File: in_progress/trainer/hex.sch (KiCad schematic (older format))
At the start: 46 parts, among them IC1 ATMEGA16-P, P12 CONN_02X08, P13 CONN_01X02, Q2 2N3904, Q3 2N3904, Q4 2N3904, Q5 2N3904, SW22 DEC/HEX, SW23 SW_PUSH, SW24 SW_PUSH, U10 JHD-162A, U8 4067, U9 ULN2803A

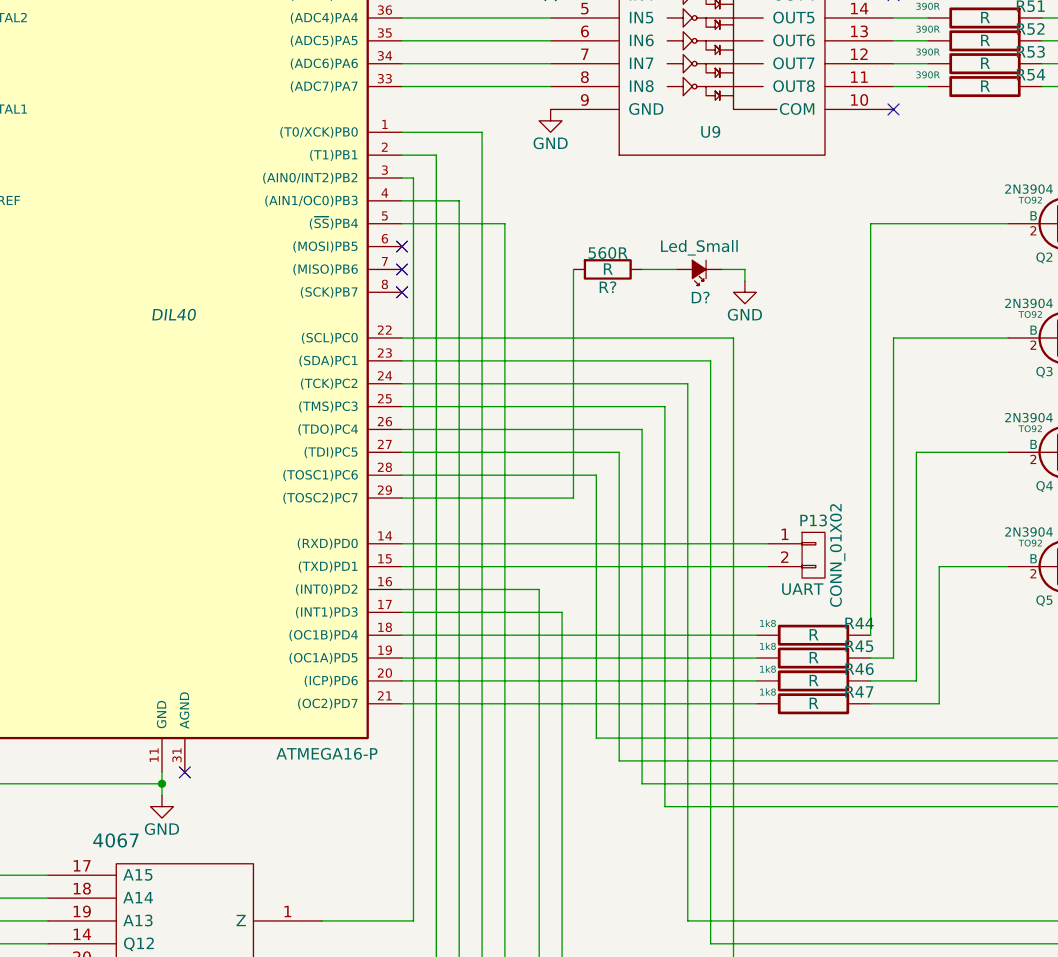
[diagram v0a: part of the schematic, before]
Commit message: .
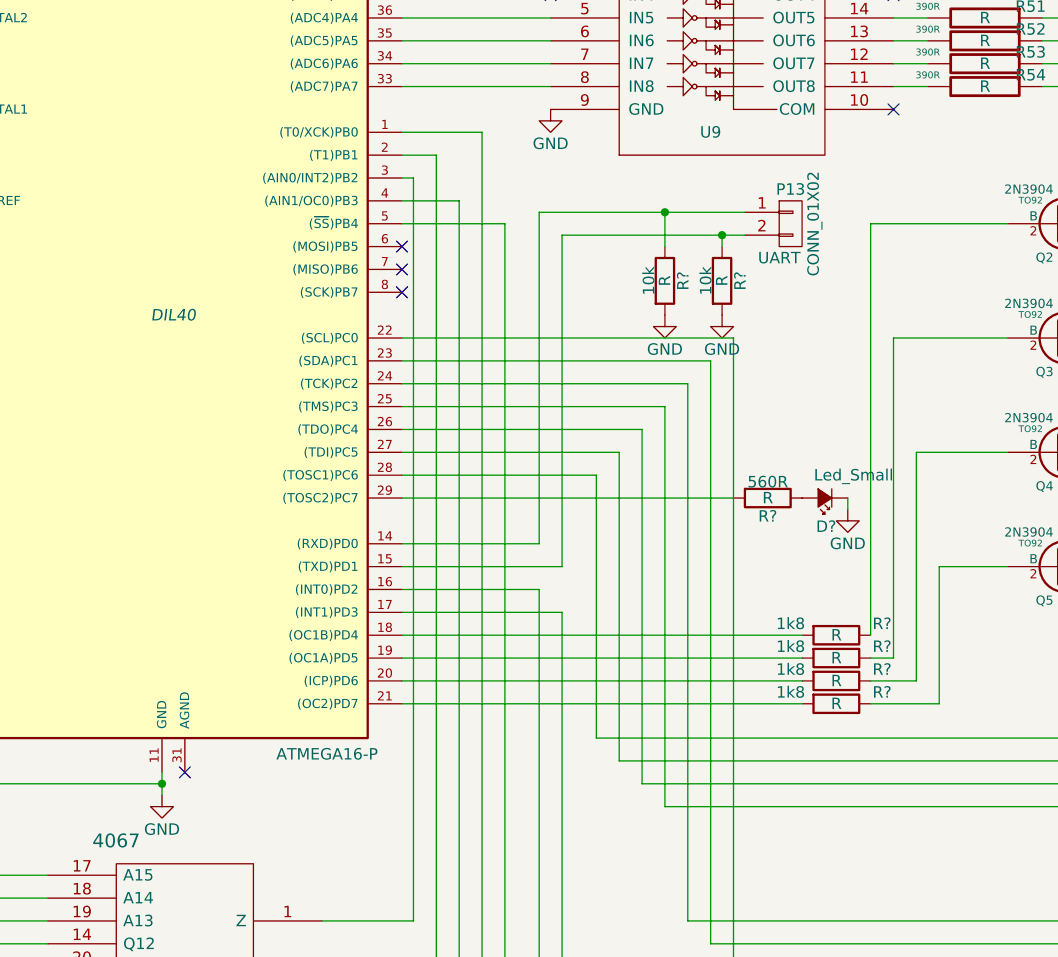
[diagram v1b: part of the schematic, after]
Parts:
- removed R44, R45, R46, R47: R, 1k8, symbol R-RESCUE-trainer
- added R? (x4): R, 1k8, symbol R
- added R? (x2): R, 10k, symbol R
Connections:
- net GND: now also R?.2, R?.2
- net at Q2.2 (B): now also R?.1
- net at IC1.18 ((OC1B)PD4): now also R?.2
- net at Q3.2 (B): now also R?.1
- net at IC1.19 ((OC1A)PD5): now also R?.2
- net at Q4.2 (B): now also R?.1
- net at IC1.20 ((ICP)PD6): now also R?.2
- net at Q5.2 (B): now also R?.1
- net at IC1.21 ((OC2)PD7): now also R?.2
- net at IC1.14 ((RXD)PD0), P13.1 (P1): now also R?.1
- net at IC1.15 ((TXD)PD1), P13.2 (P2): now also R?.1
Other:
- moved on the sheet: D?, P13, R?
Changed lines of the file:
@@
-$EndComp
-$Comp
-L R-RESCUE-trainer R44
-U 1 1 5666DBF2
-P 8400 5550
-F 0 "R44" V 8350 5750 50  0000 C CNN
-F 1 "R" V 8400 5550 50  0000 C CNN
-F 2 "1k8" V 8350 5350 30  0000 C CNN
-F 3 "" H 8400 5550 30  0000 C CNN
-	1    8400 5550
-	0    1    1    0
-$EndComp
-$Comp
-L R-RESCUE-trainer R45
-U 1 1 5666DC11
-P 8400 5650
-F 0 "R45" V 8350 5850 50  0000 C CNN
-F 1 "R" V 8400 5650 50  0000 C CNN
-F 2 "1k8" V 8350 5450 30  0000 C CNN
-F 3 "" H 8400 5650 30  0000 C CNN
-	1    8400 5650
-	0    1    1    0
-$EndComp
-$Comp
-L R-RESCUE-trainer R46
-U 1 1 5666DC17
-P 8400 5750
-F 0 "R46" V 8350 5950 50  0000 C CNN
-F 1 "R" V 8400 5750 50  0000 C CNN
-F 2 "1k8" V 8350 5550 30  0000 C CNN
-F 3 "" H 8400 5750 30  0000 C CNN
-	1    8400 5750
-	0    1    1    0
-$EndComp
-$Comp
-L R-RESCUE-trainer R47
-U 1 1 5666DC1D
-P 8400 5850
-F 0 "R47" V 8350 6050 50  0000 C CNN
-F 1 "R" V 8400 5850 50  0000 C CNN
-F 2 "1k8" V 8350 5650 30  0000 C CNN
-F 3 "" H 8400 5850 30  0000 C CNN
-	1    8400 5850
-	0    1    1    0
 $EndComp
 $Comp
@@
 L CONN_01X02 P13
 U 1 1 5669A8F7
-P 8400 5200
-F 0 "P13" H 8400 5350 50  0000 C CNN
-F 1 "CONN_01X02" V 8500 5200 50  0000 C CNN
-F 2 "UART" H 8350 5050 50  0000 C CNN
-F 3 "" H 8400 5200 50  0000 C CNN
-	1    8400 5200
+P 8300 3750
+F 0 "P13" H 8300 3900 50  0000 C CNN
+F 1 "CONN_01X02" V 8400 3750 50  0000 C CNN
+F 2 "UART" H 8250 3600 50  0000 C CNN
+F 3 "" H 8300 3750 50  0000 C CNN
+	1    8300 3750
 	1    0    0    -1
 $EndComp
@@
 	7450 6000 12100 6000
 Wire Wire Line
-	6600 4950 7350 4950
+	6600 4950 8050 4950
 Wire Wire Line
 	9400 3150 12200 3150
@@
 	6600 3650 6850 3650
 Wire Wire Line
-	6600 5150 8200 5150
-Wire Wire Line
-	6600 5250 8200 5250
-Wire Wire Line
-	6600 5550 8150 5550
-Wire Wire Line
-	6600 5650 8150 5650
-Wire Wire Line
-	6600 5750 8150 5750
-Wire Wire Line
-	6600 5850 8150 5850
+	6600 5550 8350 5550
+Wire Wire Line
+	6600 5650 8350 5650
+Wire Wire Line
+	6600 5750 8350 5750
+Wire Wire Line
+	6600 5850 8350 5850
 Wire Wire Line
 	8650 5550 8650 3750
@@
 L R R?
 U 1 1 568B24E5
-P 7500 3950
-F 0 "R?" V 7580 3950 50  0000 C CNN
-F 1 "R" V 7500 3950 50  0000 C CNN
-F 2 "560R" V 7430 3950 50  0000 C CNN
-F 3 "" H 7500 3950 50  0000 C CNN
-	1    7500 3950
+P 8200 4950
+F 0 "R?" V 8280 4950 50  0000 C CNN
+F 1 "R" V 8200 4950 50  0000 C CNN
+F 2 "560R" V 8130 4950 50  0000 C CNN
+F 3 "" H 8200 4950 50  0000 C CNN
+	1    8200 4950
 	0    1    1    0
 $EndComp
@@
 L Led_Small D?
 U 1 1 568B300A
-P 7900 3950
-F 0 "D?" H 7850 4075 50  0000 L CNN
-F 1 "Led_Small" H 7725 3850 50  0000 L CNN
-F 2 "" V 7900 3950 50  0000 C CNN
-F 3 "" V 7900 3950 50  0000 C CNN
-	1    7900 3950
+P 8450 4950
+F 0 "D?" H 8400 5075 50  0000 L CNN
+F 1 "Led_Small" H 8150 4850 50  0000 L CNN
+F 2 "" V 8450 4950 50  0000 C CNN
+F 3 "" V 8450 4950 50  0000 C CNN
+	1    8450 4950
 	-1   0    0    1
 $EndComp
@@
 L GND #PWR?
 U 1 1 568B30CE
-P 8100 4000
-F 0 "#PWR?" H 8100 3750 50  0001 C CNN
-F 1 "GND" H 8100 3850 50  0000 C CNN
-F 2 "" H 8100 4000 50  0000 C CNN
-F 3 "" H 8100 4000 50  0000 C CNN
-	1    8100 4000
-	1    0    0    -1
-$EndComp
-Wire Wire Line
-	8100 4000 8100 3950
-Wire Wire Line
-	8100 3950 8000 3950
-Wire Wire Line
-	7350 4950 7350 3950
-Wire Wire Line
-	7650 3950 7800 3950
+P 8550 5000
+F 0 "#PWR?" H 8550 4750 50  0001 C CNN
+F 1 "GND" H 8550 4850 50  0000 C CNN
+F 2 "" H 8550 5000 50  0000 C CNN
+F 3 "" H 8550 5000 50  0000 C CNN
+	1    8550 5000
+	1    0    0    -1
+$EndComp
+Wire Wire Line
+	8550 4950 8550 5000
+Wire Wire Line
+	8350 4950 8350 4950
 Wire Wire Line
 	6600 5350 7200 5350
@@
 $EndComp
 Wire Wire Line
-	5550 6250 5550 6150
+	5550 6150 5550 6250
 Wire Wire Line
 	5550 6200 4200 6200
@@
 	4200 2050 5450 2050
 Connection ~ 5450 2050
+$Comp
+L R R?
+U 1 1 568E36BE
+P 8500 5550
+F 0 "R?" V 8450 5750 50  0000 C CNN
+F 1 "R" V 8500 5550 50  0000 C CNN
+F 2 "1k8" V 8450 5350 50  0000 C CNN
+F 3 "" H 8500 5550 50  0000 C CNN
+	1    8500 5550
+	0    1    1    0
+$EndComp
+$Comp
+L R R?
+U 1 1 568E393C
+P 8500 5650
+F 0 "R?" V 8450 5850 50  0000 C CNN
+F 1 "R" V 8500 5650 50  0000 C CNN
+F 2 "1k8" V 8450 5450 50  0000 C CNN
+F 3 "" H 8500 5650 50  0000 C CNN
+	1    8500 5650
+	0    1    1    0
+$EndComp
+$Comp
+L R R?
+U 1 1 568E39D0
+P 8500 5750
+F 0 "R?" V 8450 5950 50  0000 C CNN
+F 1 "R" V 8500 5750 50  0000 C CNN
+F 2 "1k8" V 8450 5550 50  0000 C CNN
+F 3 "" H 8500 5750 50  0000 C CNN
+	1    8500 5750
+	0    1    1    0
+$EndComp
+$Comp
+L R R?
+U 1 1 568E3A67
+P 8500 5850
+F 0 "R?" V 8450 6050 50  0000 C CNN
+F 1 "R" V 8500 5850 50  0000 C CNN
+F 2 "1k8" V 8450 5650 50  0000 C CNN
+F 3 "" H 8500 5850 50  0000 C CNN
+	1    8500 5850
+	0    1    1    0
+$EndComp
+Wire Wire Line
+	6600 5150 7200 5150
+Wire Wire Line
+	7200 5150 7200 3700
+Wire Wire Line
+	7200 3700 8100 3700
+Wire Wire Line
+	6600 5250 7300 5250
+Wire Wire Line
+	7300 5250 7300 3800
+Wire Wire Line
+	7300 3800 8100 3800
+$Comp
+L R R?
+U 1 1 568E50BC
+P 7750 4000
+F 0 "R?" V 7830 4000 50  0000 C CNN
+F 1 "R" V 7750 4000 50  0000 C CNN
+F 2 "10k" V 7680 4000 50  0000 C CNN
+F 3 "" H 7750 4000 50  0000 C CNN
+	1    7750 4000
+	1    0    0    -1
+$EndComp
+$Comp
+L R R?
+U 1 1 568E51CB
+P 8000 4000
+F 0 "R?" V 8080 4000 50  0000 C CNN
+F 1 "R" V 8000 4000 50  0000 C CNN
+F 2 "10k" V 7930 4000 50  0000 C CNN
+F 3 "" H 8000 4000 50  0000 C CNN
+	1    8000 4000
+	1    0    0    -1
+$EndComp
+$Comp
+L GND #PWR?
+U 1 1 568E5271
+P 7750 4150
+F 0 "#PWR?" H 7750 3900 50  0001 C CNN
+F 1 "GND" H 7750 4000 50  0000 C CNN
+F 2 "" H 7750 4150 50  0000 C CNN
+F 3 "" H 7750 4150 50  0000 C CNN
+	1    7750 4150
+	1    0    0    -1
+$EndComp
+$Comp
+L GND #PWR?
+U 1 1 568E530C
+P 8000 4150
+F 0 "#PWR?" H 8000 3900 50  0001 C CNN
+F 1 "GND" H 8000 4000 50  0000 C CNN
+F 2 "" H 8000 4150 50  0000 C CNN
+F 3 "" H 8000 4150 50  0000 C CNN
+	1    8000 4150
+	1    0    0    -1
+$EndComp
+Wire Wire Line
+	7750 3850 7750 3700
+Connection ~ 7750 3700
+Wire Wire Line
+	8000 3850 8000 3800
+Connection ~ 8000 3800
 $EndSCHEMATC
